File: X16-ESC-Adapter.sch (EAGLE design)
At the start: 9 parts

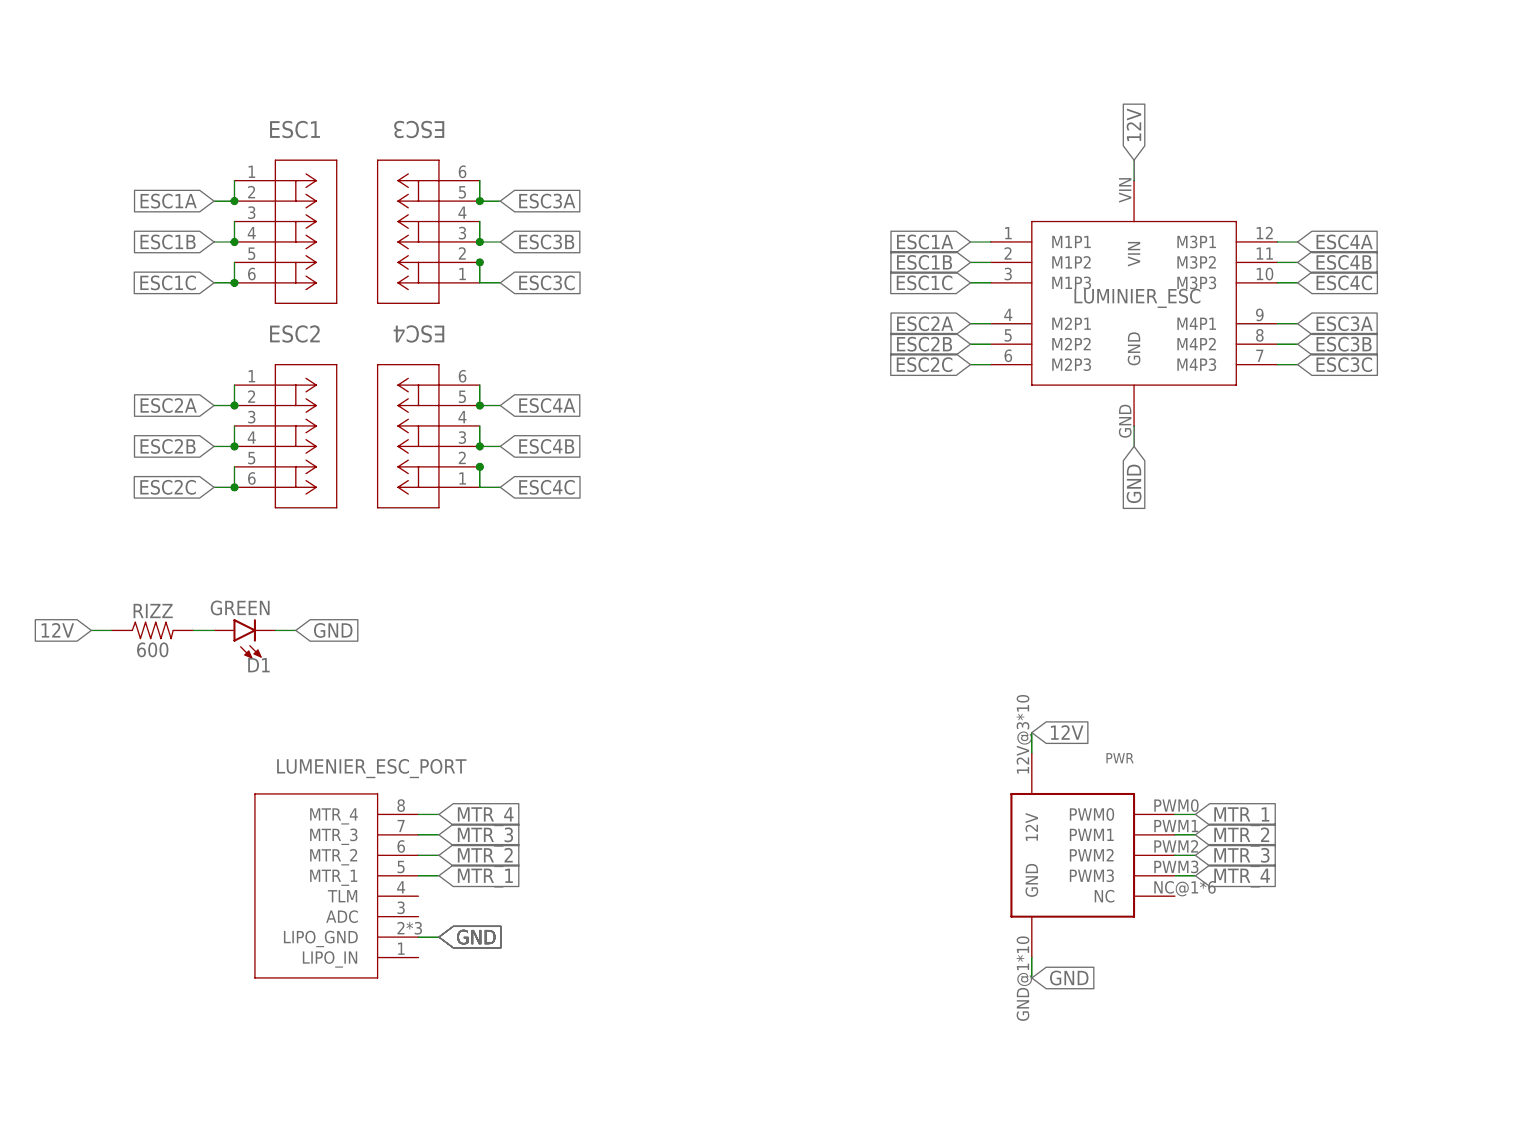
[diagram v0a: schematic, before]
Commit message: Update X16-ESC-Adapter.sch
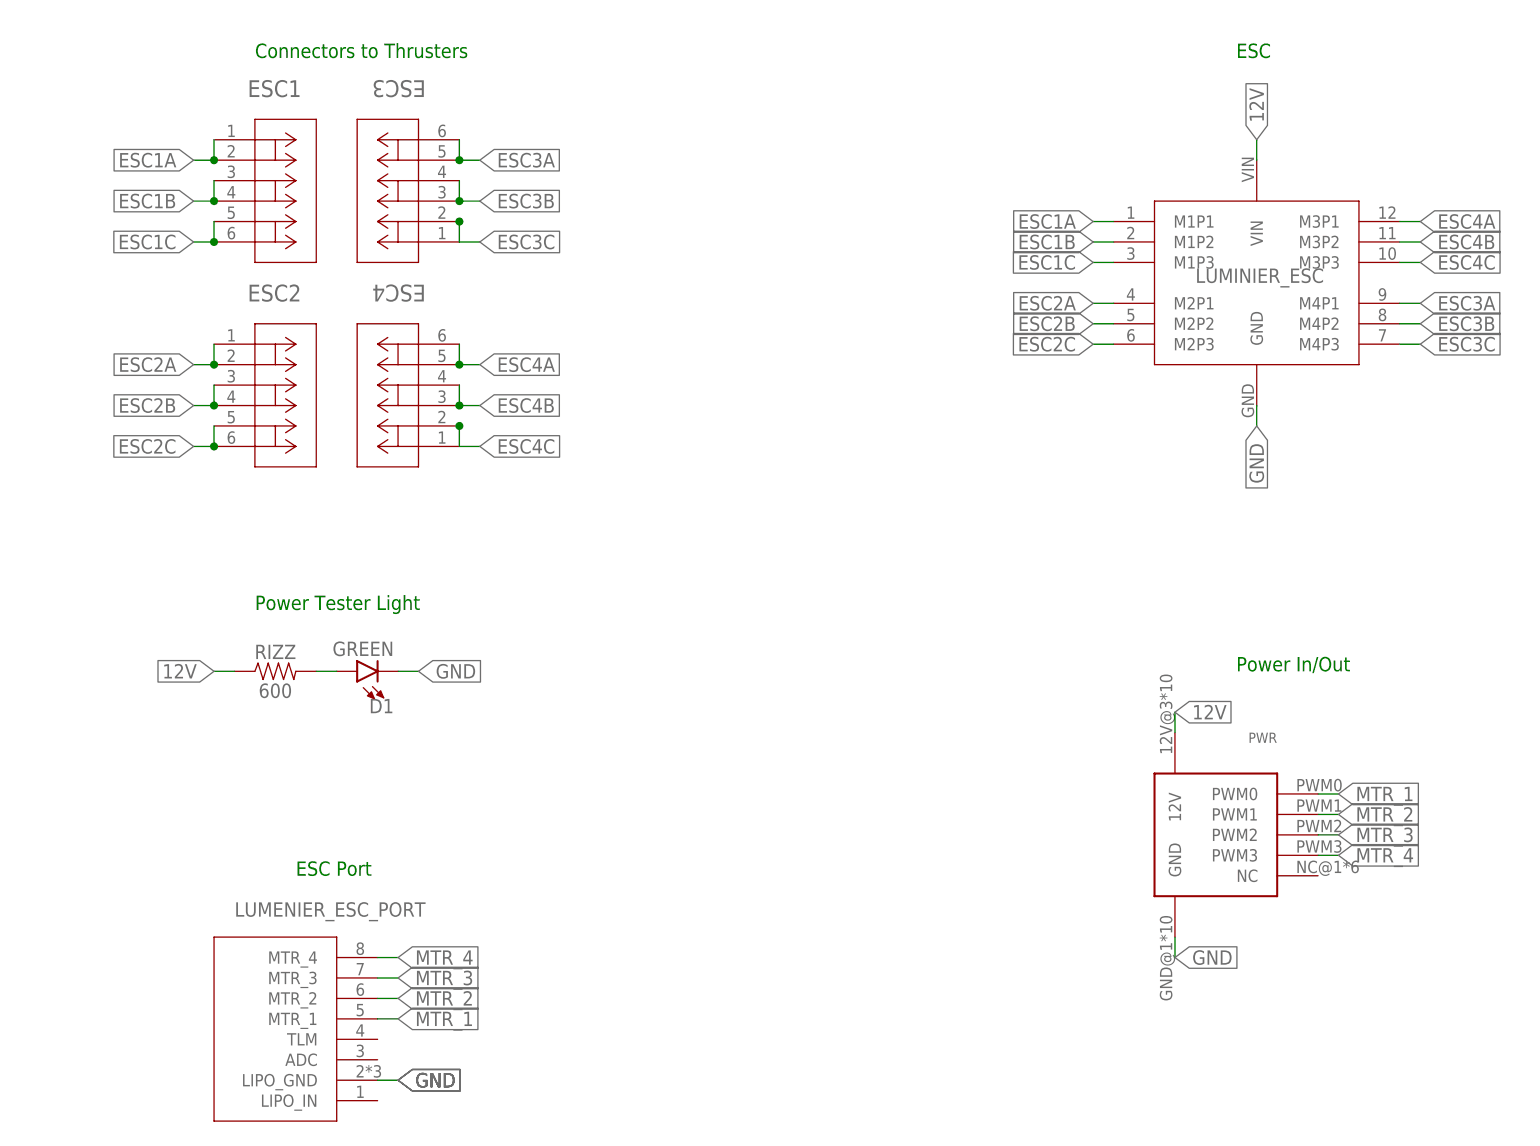
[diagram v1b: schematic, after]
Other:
- note added: "Connectors to Thrusters"
- note added: "ESC"
- note added: "ESC Port"
- note added: "Power In/Out"
- note added: "Power Tester Light"
- moved on the sheet: D1, ESC1, ESC2, ESC3, ESC4, LUMENIER_ESC_PORT, LUMINIER_ESC, PWR, RIZZ

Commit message: First set of changes after alumni design review
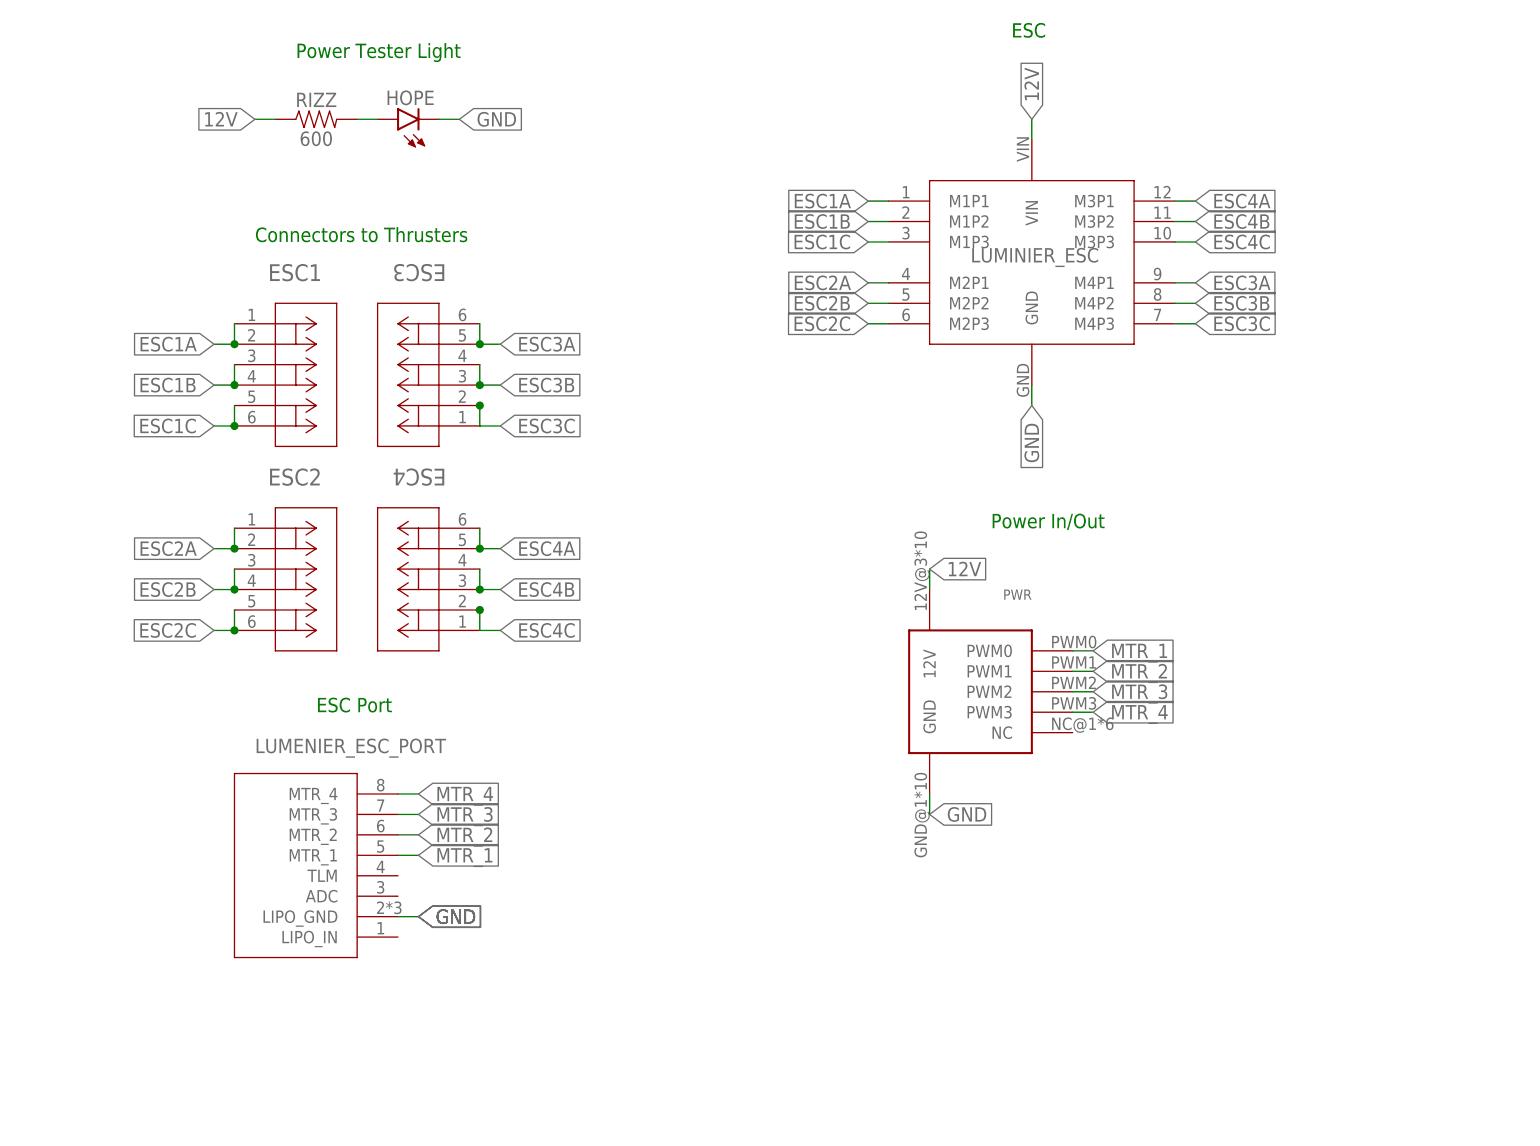
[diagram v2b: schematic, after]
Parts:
- removed D1: GREEN, SparkFun-LED:LED0603
- added HOPE: (no value), led:LEDCHIPLED_0805
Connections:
- net GND: now also HOPE.C; no longer D1.C
- net N$1: now also HOPE.A; no longer D1.A
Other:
- moved on the sheet: ESC1, ESC2, ESC3, ESC4, LUMENIER_ESC_PORT, LUMINIER_ESC, PWR, RIZZ

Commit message: Updated (11/4)
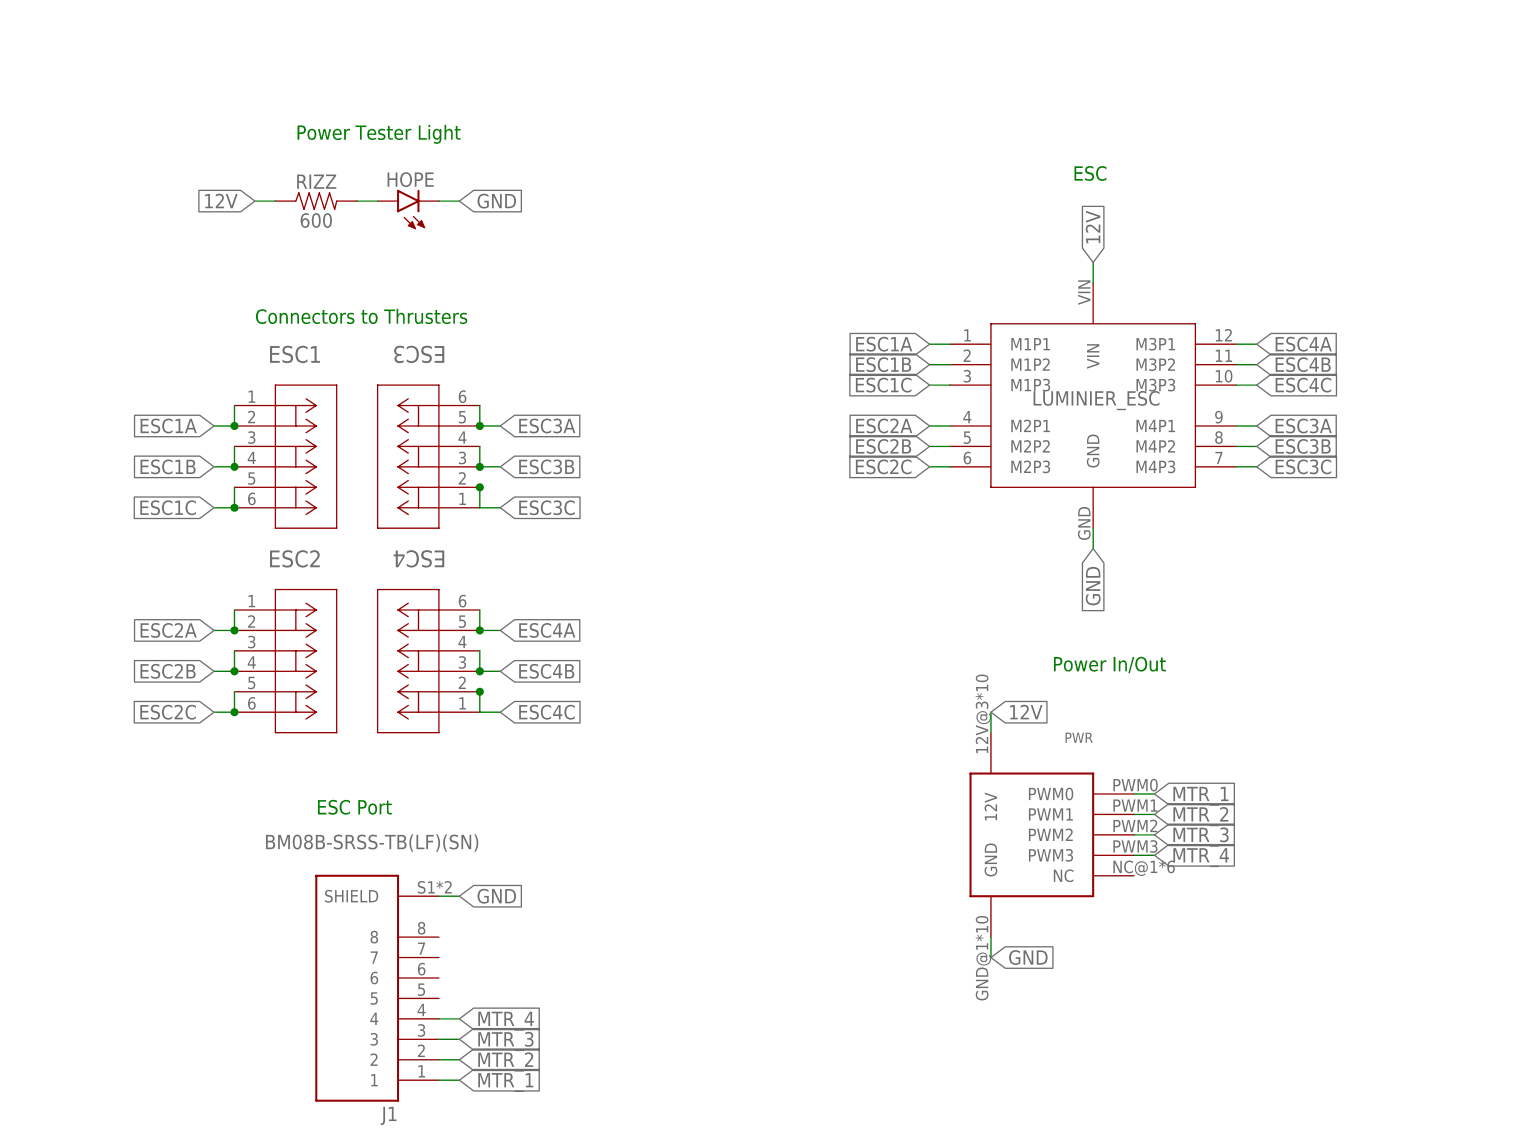
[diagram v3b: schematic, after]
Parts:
- removed LUMENIER_ESC_PORT: CONN_JST_8_PIN, X16-ESC-Adapter:CONN_JST_8_PIN
- added J1: BM08B-SRSS-TB(LF)(SN), X16-ESC-Adapter:BM08B-SRSS-TB(LF)(SN)
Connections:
- net GND: now also J1.SHIELD; no longer LUMENIER_ESC_PORT.LIPO_GND
- net MTR_1: now also J1.1; no longer LUMENIER_ESC_PORT.MTR_1
- net MTR_2: now also J1.2; no longer LUMENIER_ESC_PORT.MTR_2
- net MTR_3: now also J1.3; no longer LUMENIER_ESC_PORT.MTR_3
- net MTR_4: now also J1.4; no longer LUMENIER_ESC_PORT.MTR_4
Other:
- moved on the sheet: ESC1, ESC2, ESC3, ESC4, HOPE, LUMINIER_ESC, PWR, RIZZ
